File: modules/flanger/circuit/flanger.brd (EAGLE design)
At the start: 100 x 80 mm, 28 parts, among them IC1 LM324N, U1 ATTINY84

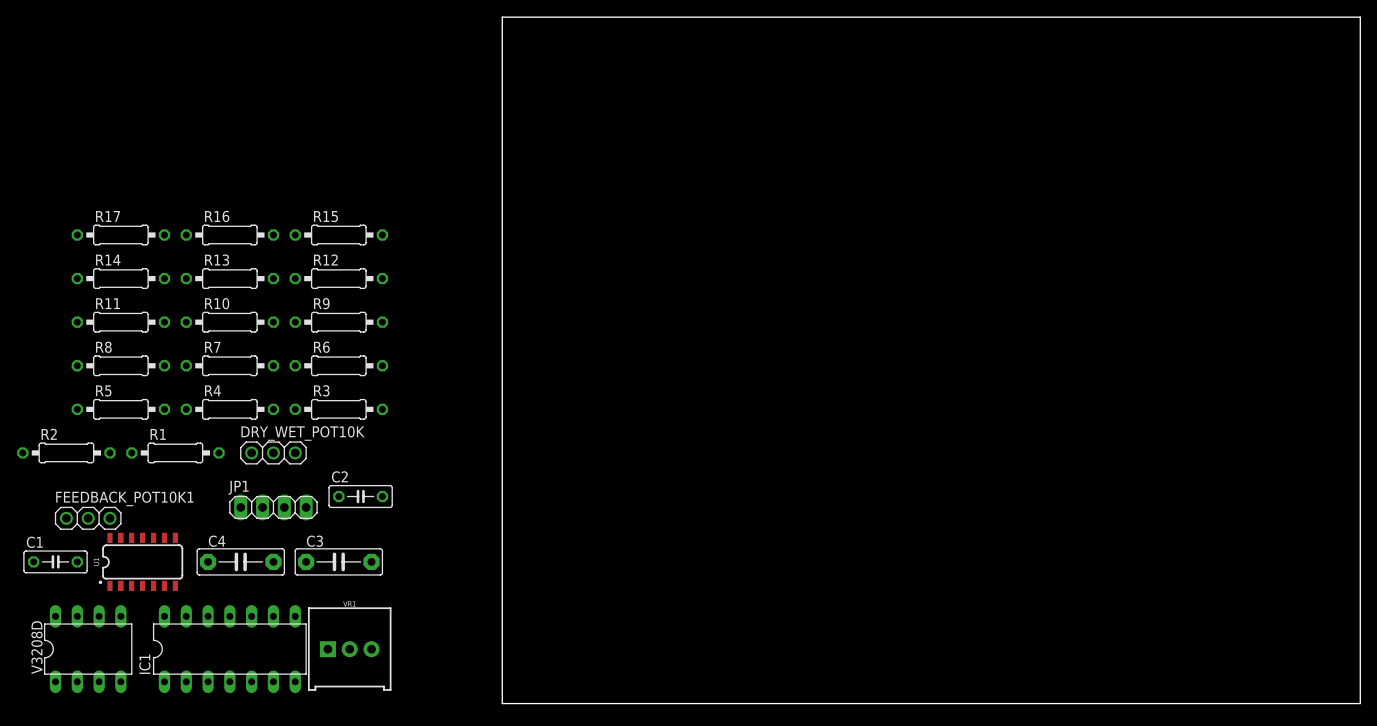
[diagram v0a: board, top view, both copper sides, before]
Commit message: flanger
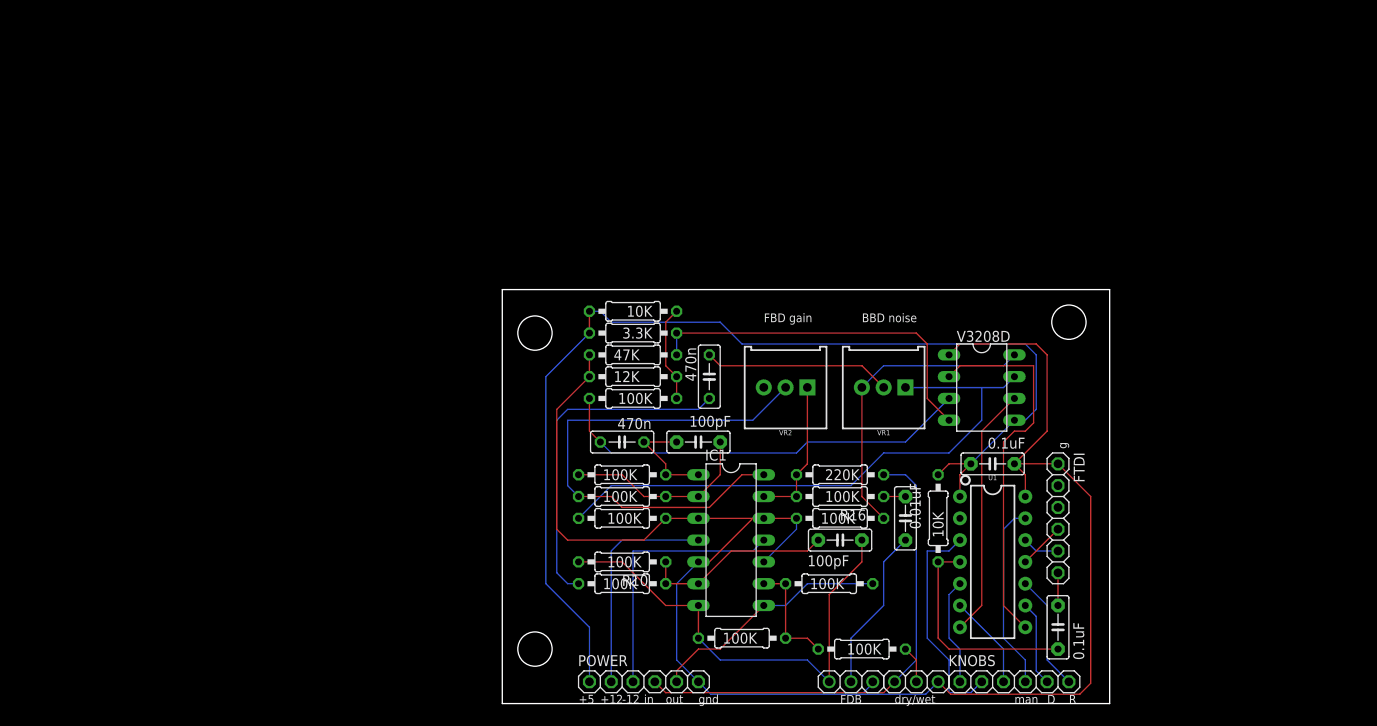
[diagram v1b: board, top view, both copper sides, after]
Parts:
- removed JP1: (no value), pinhead:1X04
- removed R12: 100K, rcl:0207/10
- added C5: 0.01uF, capacitor-wima:C5B2.5
- added C6, C7: 0.1uF, capacitor-wima:C5B2.5
- added FTDI, KNOBS, POWER: (no value), adafruit:1X06
- added R18: 10K, rcl:0207/10
- added VR2: 100k, SparkFun-Resistors:TRIMPOT-PTH-3386U
- C3, C4: device capacitor-wima:C7.5B3 -> capacitor-wima:C5B2.5
- R15: value 100K -> 220K
- U1: value ATTINY84 -> ATTINY84ATTINY84-20PU; device SparkFun-IC-Microcontroller:SO14 -> SparkFun-IC-Microcontroller:DIP14
- moved V3208D 108.5 mm to (55.9, 36.8), turned to 270 degrees
- moved U1 99.1 mm to (57.1, 16.5), turned to 270 degrees
- moved R17 98.9 mm to (41.9, 6.35), turned to 180 degrees
- moved FEEDBACK_POT10K1 90.9 mm to (40.6, 2.54)
- moved R14 83.6 mm to (27.9, 7.62)
- moved DRY_WET_POT10K 79.5 mm to (48.3, 2.54), turned to 180 degrees
- moved R13 78.4 mm to (38.1, 14.0)
- moved R16 77.4 mm to (39.4, 24.1), turned to 180 degrees
- moved C4 69.9 mm to (39.4, 19.1)
- moved VR1 69.3 mm to (44.5, 36.8), turned to 180 degrees
- moved C1 67.5 mm to (14.0, 30.5), turned to 180 degrees
- moved R2 66.3 mm to (15.2, 35.6), turned to 180 degrees
- moved R11 65.9 mm to (14.0, 14.0)
- moved R15 64.8 mm to (39.4, 26.7), turned to 180 degrees
- moved R6 61.1 mm to (39.4, 21.6)
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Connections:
- new net DEPTH: KNOBS.5, U1.9
- new net MANUAL: KNOBS.4, U1.13
- new net N$14: C5.2, R16.1
- new net N$16: C7.1, R18.1, U1.4
- new net RATE: KNOBS.6, U1.10
- new net RESET: C7.2, FTDI.6
- new net RX: FTDI.5, U1.12
- new net SPARE1: KNOBS.1, U1.5
- new net SPARE2: KNOBS.2, U1.3
- new net SPARE3: KNOBS.3, U1.6
- new net TX: FTDI.4, U1.11
- net +12V: now also POWER.2
- net +5V: now also C6.2, POWER.1, R18.2, U1.1
- net -12V: now also POWER.3
- net CLK1: now also U1.8; no longer U1.6
- net GND: now also C6.1, FTDI.1, POWER.6, U1.14
- net N$11: now also VR2.2; no longer R12.2
- net N$15: now also C5.1; no longer R16.1
- net N$7: now also VR2.1; no longer R12.1
- net SIGNAL_IN: now also POWER.4
- net SIGNAL_OUT: now also POWER.5
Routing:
- net GND: track 0.00 -> 197.2 mm
- net +5V: track 0.00 -> 126.8 mm
- net N$2: track 0.00 -> 68.8 mm
- net N$11: track 0.00 -> 60.1 mm
- net SIGNAL_IN: track 0.00 -> 57.2 mm
- net N$12: track 0.00 -> 55.3 mm
- net N$3: track 0.00 -> 49.4 mm
- net CLK1: track 0.00 -> 44.1 mm
- net N$6: track 0.00 -> 42.2 mm
- net BBD_OUT: track 0.00 -> 39.7 mm
- net N$1: track 0.00 -> 35.7 mm
- net -12V: track 0.00 -> 31.0 mm
- net CLK2: track 0.00 -> 29.3 mm
- net SIGNAL_OUT: track 0.00 -> 28.3 mm
- net SPARE2: track 0.00 -> 26.2 mm
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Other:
- board size 100 x 80 mm -> 70.8 x 48.2 mm
- board text added: "+12"
- board text added: "+5"
- board text added: "-12"
- board text added: "BBD Delay/Flanger"
- board text added: "BBD noise"
- board text added: "D"
- board text added: "DUMAIS"
- board text added: "FBD gain"
- board text added: "FDB"
- board text added: "R"
- board text added: "dry/wet"
- board text added: "g"
- board text added: "gnd"
- board text added: "in"
- board text added: "man"
- board text added: "out"
